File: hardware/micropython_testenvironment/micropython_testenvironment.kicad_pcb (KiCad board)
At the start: 2 copper layers, 80 x 100 mm, 5 parts, among them J102 Conn_02x20_Odd_Even, J104 Conn_02x20_Odd_Even, U101 ESP32-C3-WROOM-02, U102 Pico, U103 Seeed Studio XIAO SAMD21

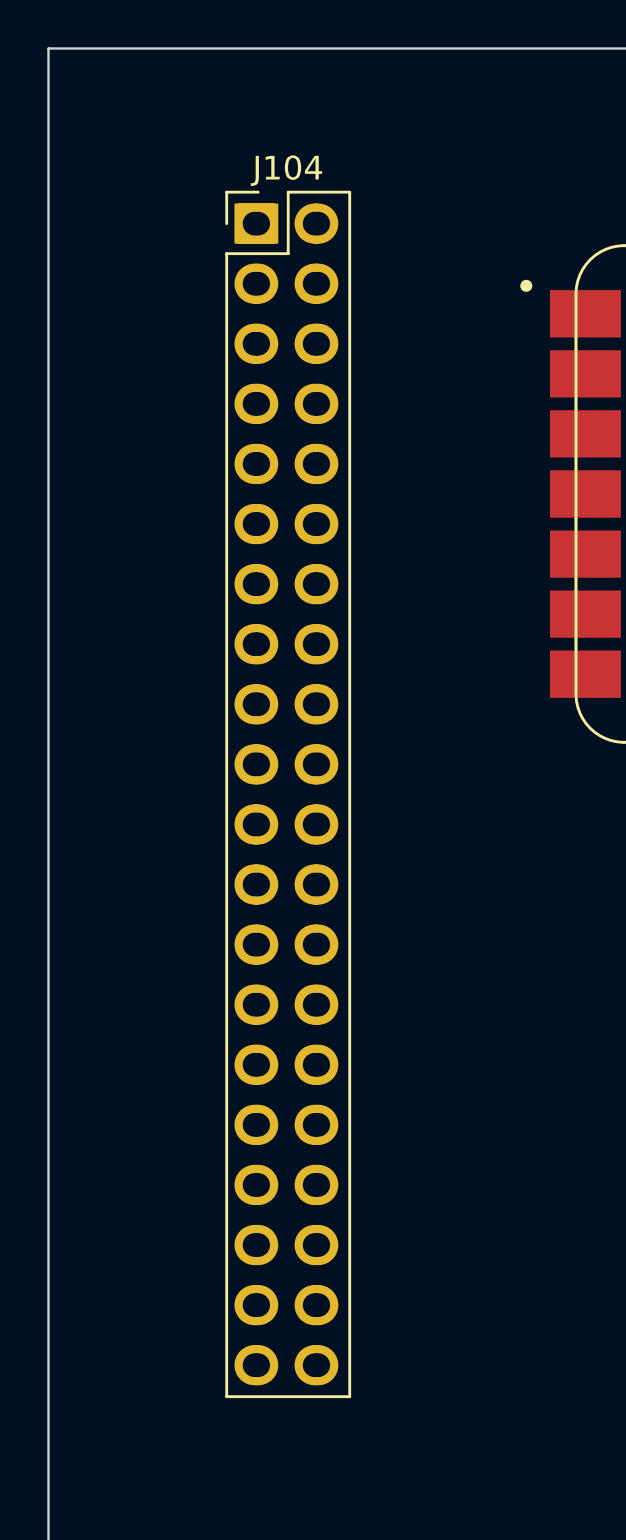
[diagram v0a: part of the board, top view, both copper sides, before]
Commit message: RPi_Hat
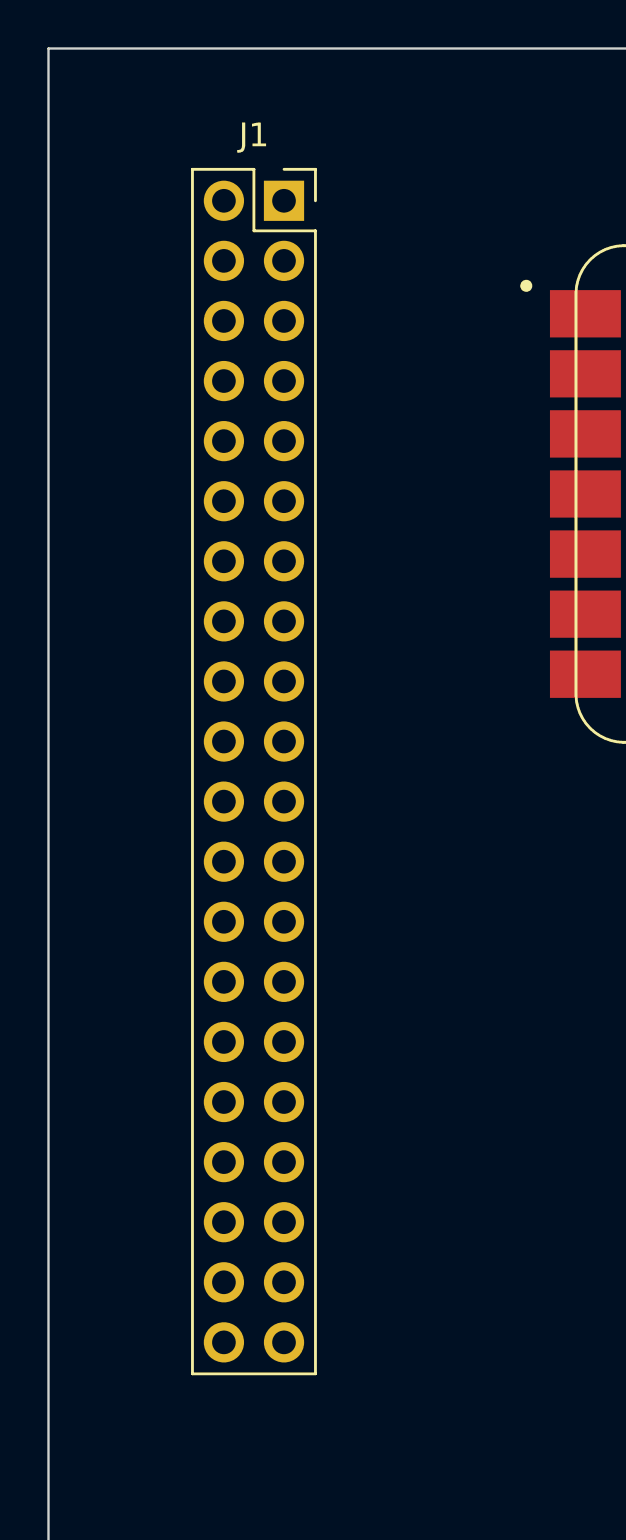
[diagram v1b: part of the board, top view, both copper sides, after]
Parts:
- removed J102: Conn_02x20_Odd_Even, Connector_PinSocket_2.54mm:PinSocket_2x20_P2.54mm_Vertical
- removed J104: Conn_02x20_Odd_Even, Connector_PinHeader_2.54mm:PinHeader_2x20_P2.54mm_Vertical
- added J1: RPi_GPIO, 00_project_RPI_Hat:PinSocket_2x20_P2.54mm_Vertical-stackable, F.Cu at (110.0, 56.4)

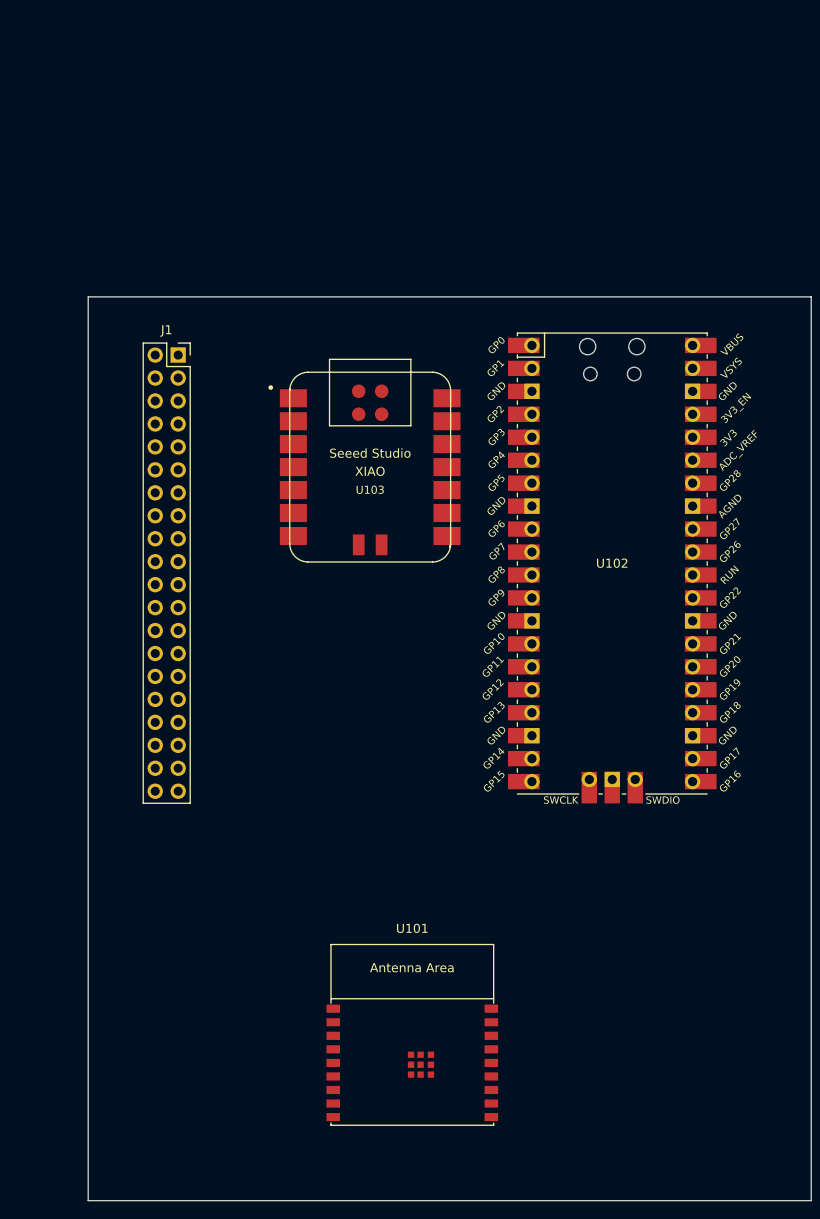
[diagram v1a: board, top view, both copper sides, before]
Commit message: RPi_Hat 2
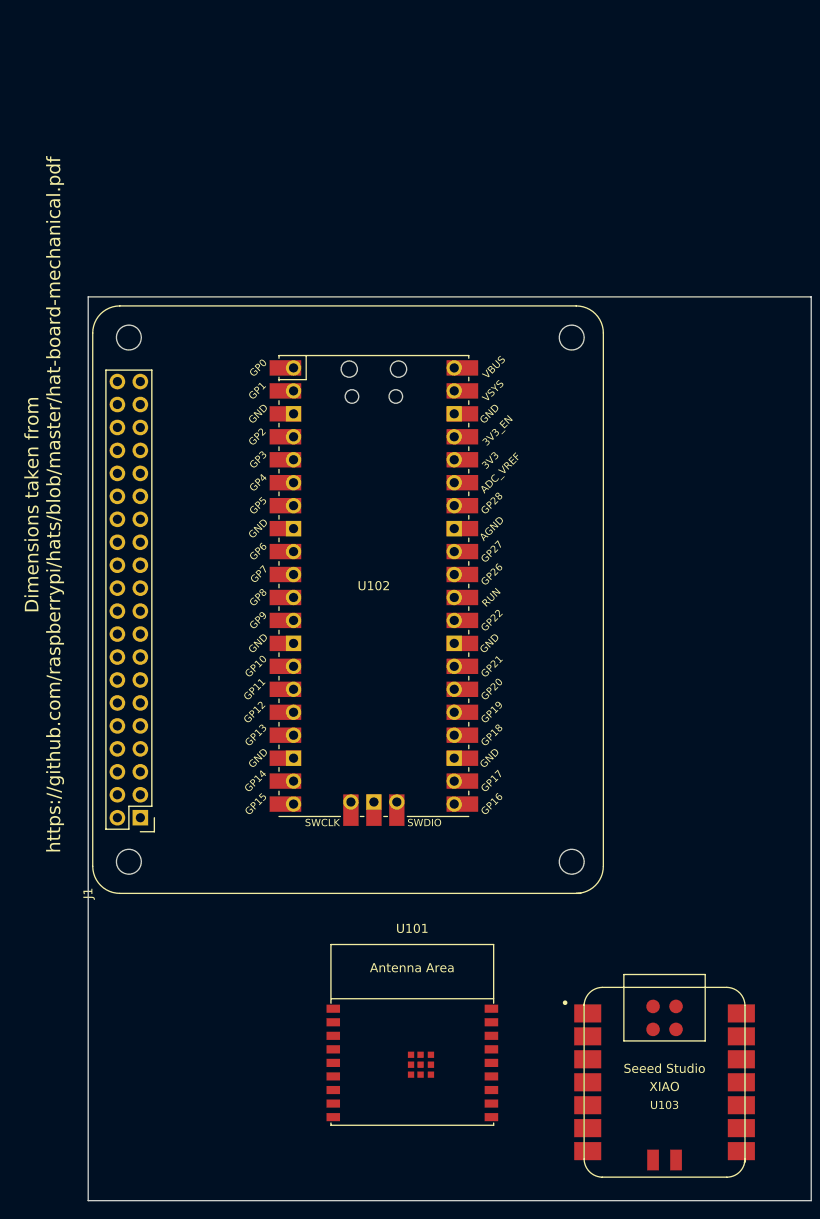
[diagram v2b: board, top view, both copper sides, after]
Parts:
- J1: footprint 00_project_RPI_Hat:PinSocket_2x20_P2.54mm_Vertical-stackable -> 00_project_RPI_Hat:RPi_Hat
- moved U103 75.5 mm to (163.8, 136.9)
- moved J1 60.3 mm to (100.5, 116.0), turned to 90 degrees
- moved U102 26.5 mm to (131.6, 82.0)

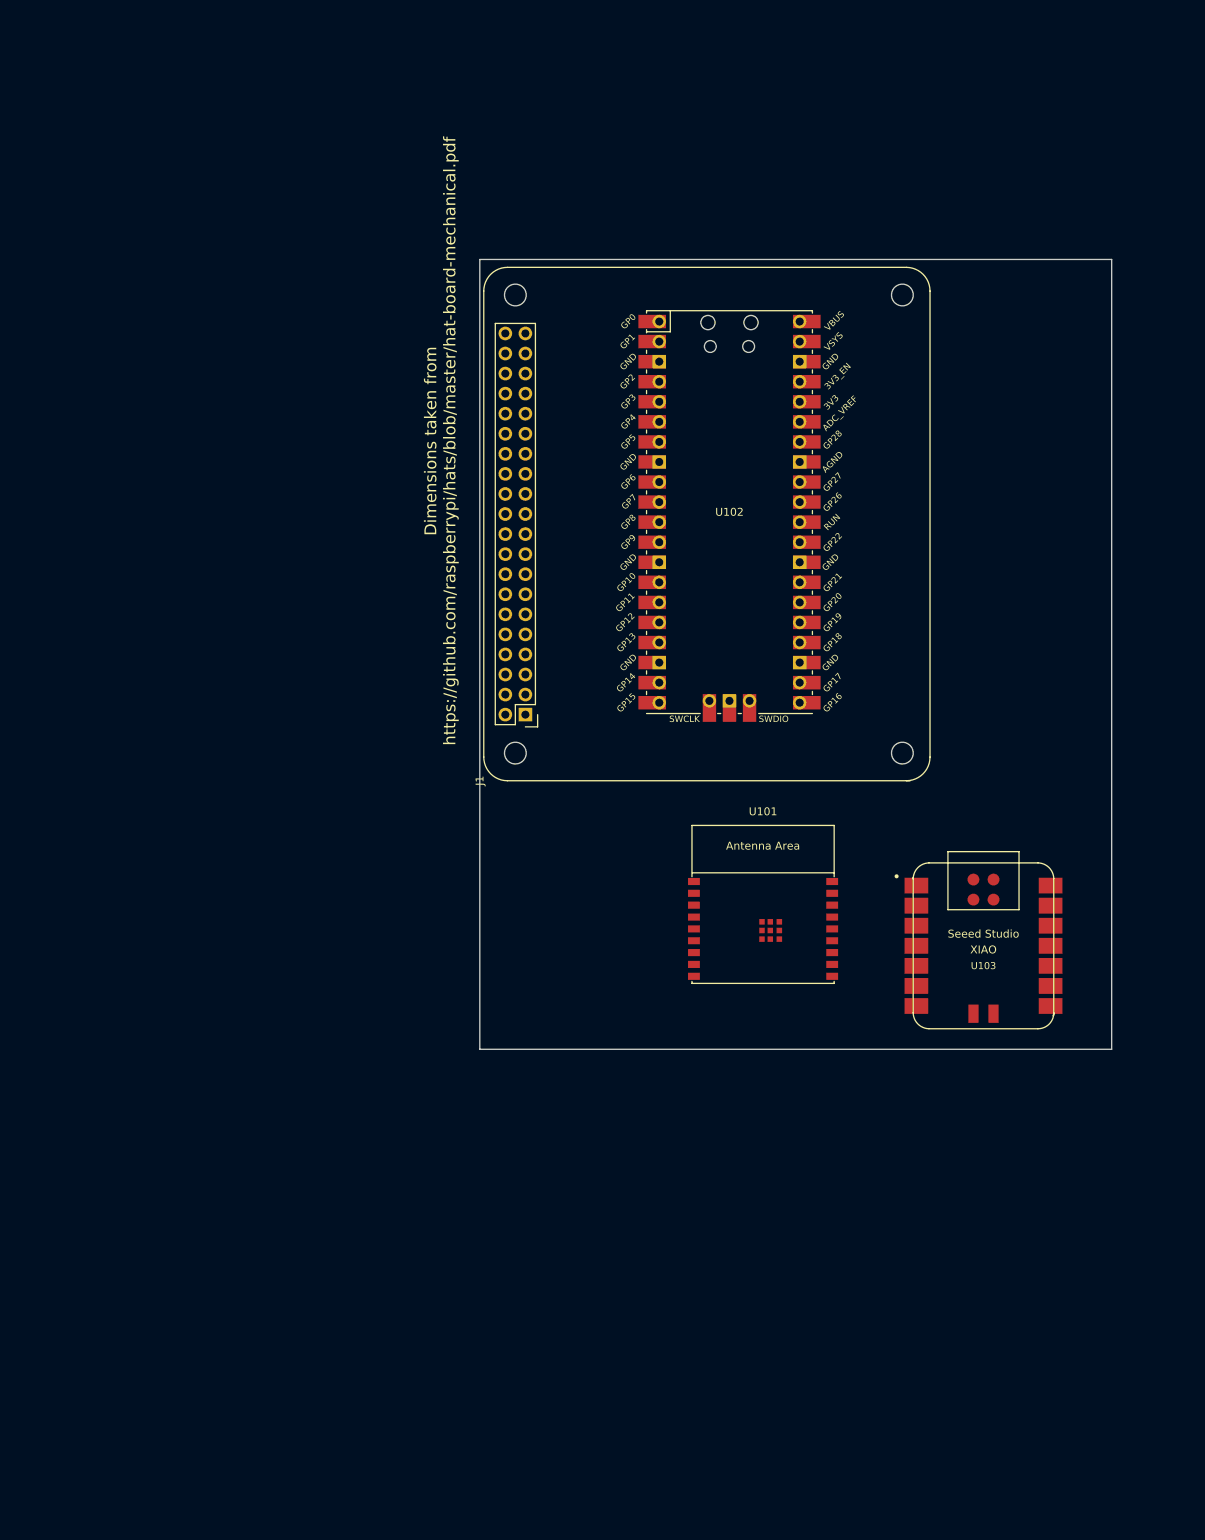
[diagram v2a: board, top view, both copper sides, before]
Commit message: Some documentation
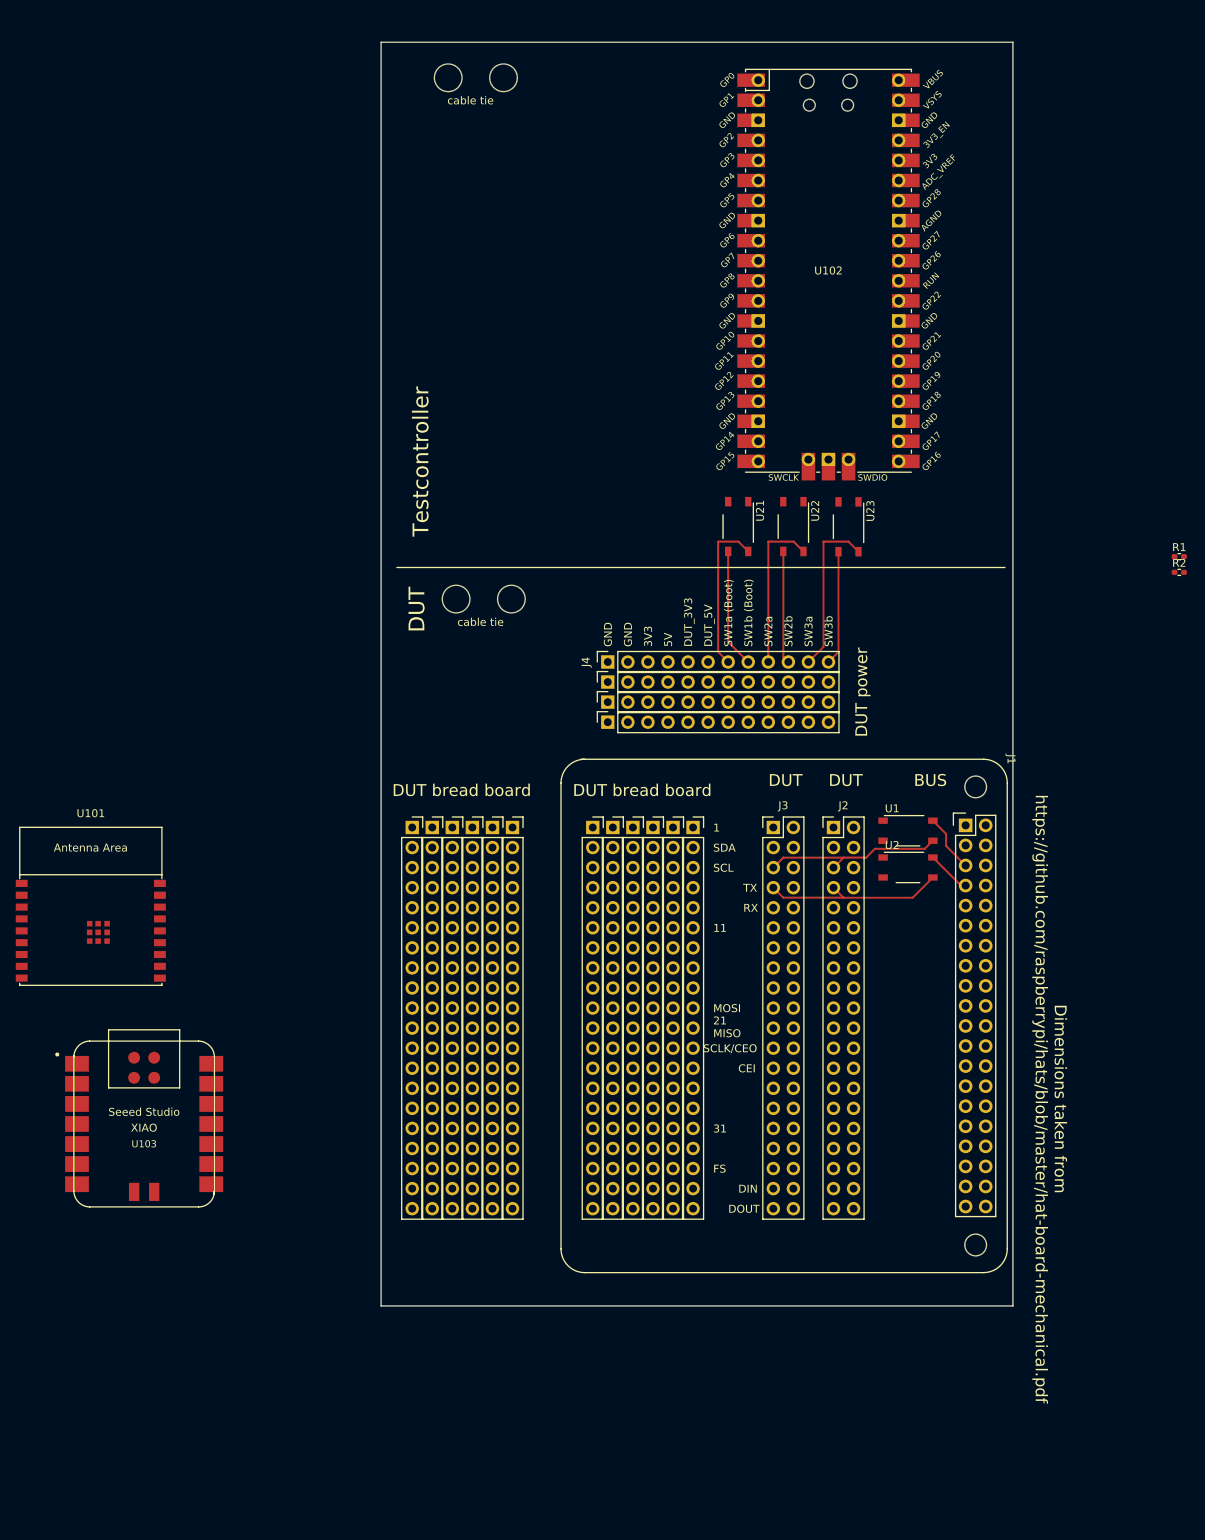
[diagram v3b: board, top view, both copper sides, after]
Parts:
- added J1000: Conn_01x20, Connector_PinSocket_2.54mm:PinSocket_1x20_P2.54mm_Vertical, F.Cu at (99.1, 121.9)
- added J1000: Conn_01x20, Connector_PinSocket_2.54mm:PinSocket_1x20_P2.54mm_Vertical, F.Cu at (119.4, 121.9)
- added J1000: Conn_01x20, Connector_PinSocket_2.54mm:PinSocket_1x20_P2.54mm_Vertical, F.Cu at (121.9, 121.9)
- added J1000: Conn_01x20, Connector_PinSocket_2.54mm:PinSocket_1x20_P2.54mm_Vertical, F.Cu at (94.0, 121.9)
- added J1000: Conn_01x12, Connector_PinSocket_2.54mm:PinSocket_1x12_P2.54mm_Vertical, F.Cu at (116.2, 103.5)
- added J1000: Conn_01x20, Connector_PinSocket_2.54mm:PinSocket_1x20_P2.54mm_Vertical, F.Cu at (101.6, 121.9)
- added J1000: Conn_01x20, Connector_PinSocket_2.54mm:PinSocket_1x20_P2.54mm_Vertical, F.Cu at (127.0, 121.9)
- added J1000: Conn_01x12, Connector_PinSocket_2.54mm:PinSocket_1x12_P2.54mm_Vertical, F.Cu at (116.2, 106.0)
- added J1000: Conn_01x20, Connector_PinSocket_2.54mm:PinSocket_1x20_P2.54mm_Vertical, F.Cu at (104.1, 121.9)
- added J1000: Conn_01x20, Connector_PinSocket_2.54mm:PinSocket_1x20_P2.54mm_Vertical, F.Cu at (96.5, 121.9)
- added J1000: Conn_01x20, Connector_PinSocket_2.54mm:PinSocket_1x20_P2.54mm_Vertical, F.Cu at (124.5, 121.9)
- added J1000: Conn_01x20, Connector_PinSocket_2.54mm:PinSocket_1x20_P2.54mm_Vertical, F.Cu at (116.8, 121.9)
- added J1000: Conn_01x20, Connector_PinSocket_2.54mm:PinSocket_1x20_P2.54mm_Vertical, F.Cu at (91.4, 121.9)
- added J1000: Conn_01x12, Connector_PinSocket_2.54mm:PinSocket_1x12_P2.54mm_Vertical, F.Cu at (116.2, 108.6)
- added J1000: Conn_01x20, Connector_PinSocket_2.54mm:PinSocket_1x20_P2.54mm_Vertical, F.Cu at (114.3, 121.9)
- added J2: Conn_01x20, 00_project_library:PinSocket_2x20_P2.54mm_Vertical-mirrored, F.Cu at (147.3, 121.9)
- added J3: Conn_01x20, 00_project_library:PinSocket_2x20_P2.54mm_Vertical-mirrored-bare, F.Cu at (139.7, 121.9)
- added J4: Conn_01x12, Connector_PinSocket_2.54mm:PinSocket_1x12_P2.54mm_Vertical, F.Cu at (116.2, 101.0)
- added R1: 470R, Resistor_SMD:R_0402_1005Metric_Pad0.72x0.64mm_HandSolder, F.Cu at (188.6, 87.6)
- added R2: 470R, Resistor_SMD:R_0402_1005Metric_Pad0.72x0.64mm_HandSolder, F.Cu at (188.6, 89.6)
- added REF**: MountingHole_3.5mm, MountingHole:MountingHole_3.5mm, F.Cu at (104.0, 93.0)
- added REF**: MountingHole_3.5mm, MountingHole:MountingHole_3.5mm, F.Cu at (96.0, 27.0)
- added REF**: MountingHole_3.5mm, MountingHole:MountingHole_3.5mm, F.Cu at (103.0, 27.0)
- added REF**: MountingHole_3.5mm, MountingHole:MountingHole_3.5mm, F.Cu at (97.0, 93.0)
- added U1: TLP172GM, Package_SO:MFSOP6-4_4.4x3.6mm_P1.27mm, F.Cu at (154.2, 122.3)
- added U2: TLP172GM, Package_SO:MFSOP6-4_4.4x3.6mm_P1.27mm, F.Cu at (154.2, 127.0)
- added U21: TLP172GM, Package_SO:MFSOP6-4_4.4x3.6mm_P1.27mm, F.Cu at (132.7, 83.8)
- added U22: TLP172GM, Package_SO:MFSOP6-4_4.4x3.6mm_P1.27mm, F.Cu at (139.7, 83.8)
- added U23: TLP172GM, Package_SO:MFSOP6-4_4.4x3.6mm_P1.27mm, F.Cu at (146.7, 83.8)
- J1: footprint 00_project_RPI_Hat:RPi_Hat -> 00_project_RPI_Hat:RPi_Hat_2holes
- moved U103 108.6 mm to (57.5, 159.5)
- moved U101 85.1 mm to (50.8, 134.9)
- moved J1 66.3 mm to (166.8, 113.3), turned to -90 degrees
- moved U102 33.0 mm to (144.1, 51.4)
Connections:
- J1 pad 10: unconnected-(J1-BCM15_RXD-Pad10) -> BUS_10
- J1 pad 11: unconnected-(J1-BCM17-Pad11) -> BUS_11
- J1 pad 13: unconnected-(J1-BCM27-Pad13) -> BUS_13
- J1 pad 15: unconnected-(J1-BCM22-Pad15) -> BUS_15
- J1 pad 5: unconnected-(J1-BCM3_SCL-Pad5) -> BUS_5
- J1 pad 7: unconnected-(J1-BCM4_GPCLK0-Pad7) -> BUS_7
- J1 pad 8: unconnected-(J1-BCM14_TXD-Pad8) -> BUS_8
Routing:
- net DUT_7: track 0.00 -> 23.6 mm
- net DUT_5: track 0.00 -> 23.4 mm
- net SW3a: track 0.00 -> 21.0 mm
- net SW2a: track 0.00 -> 20.2 mm
- net SW1a (Boot): track 0.00 -> 20.1 mm
- net SW1b (Boot): track 0.00 -> 15.0 mm
- net SW3b: track 0.00 -> 14.5 mm
- net SW2b: track 0.00 -> 14.3 mm
- net BUS_5: track 0.00 -> 7.39 mm
- net BUS_7: track 0.00 -> 5.62 mm
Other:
- board size 80 x 100 mm -> 80 x 160 mm
- board text added: "1"
- board text added: "11"
- board text added: "21 MISO"
- board text added: "31"
- board text added: "3V3"
- board text added: "5V"
- board text added: "BUS"
- board text added: "CEI"
- board text added: "DIN"
- board text added: "DOUT"
- board text added: "DUT"
- board text added: "DUT bread board"
- board text added: "DUT power"
- board text added: "DUT_3V3"
- board text added: "DUT_5V"
- board text added: "FS"
- board text added: "GND"
- board text added: "MOSI"
- board text added: "RX"
- board text added: "SCL"
- board text added: "SCLK/CEO"
- board text added: "SDA"
- board text added: "SW1a (Boot)"
- board text added: "SW1b (Boot)"
- board text added: "SW2a"
- board text added: "SW2b"
- board text added: "SW3a"
- board text added: "SW3b"
- board text added: "TX"
- board text added: "Testcontroller"
- board text added: "cable tie"
